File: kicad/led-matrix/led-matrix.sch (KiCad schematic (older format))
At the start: 4 parts

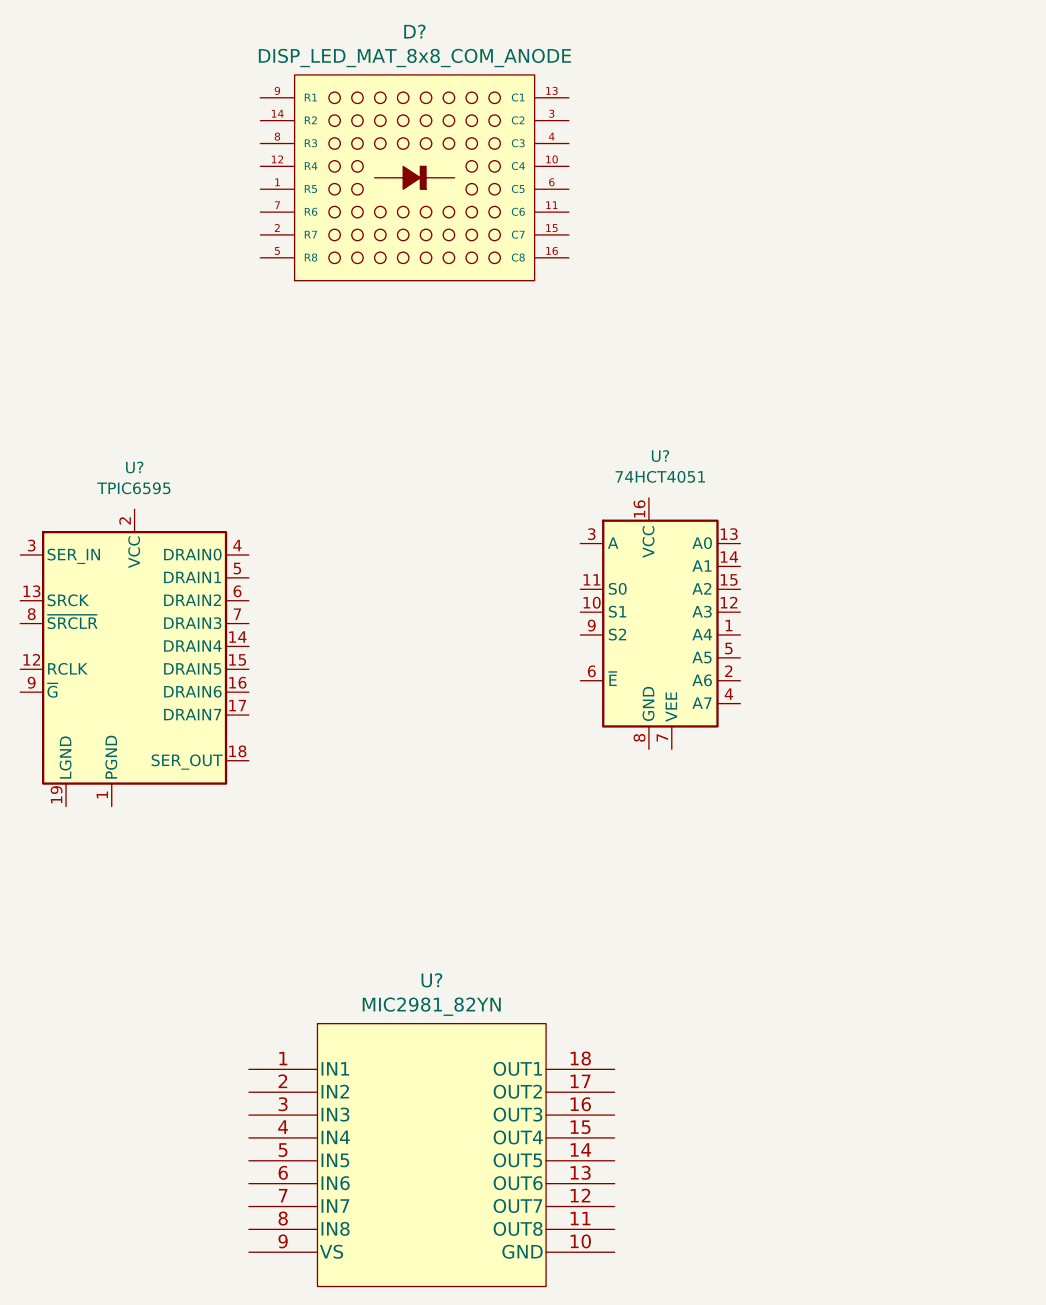
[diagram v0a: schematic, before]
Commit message: Update schematix
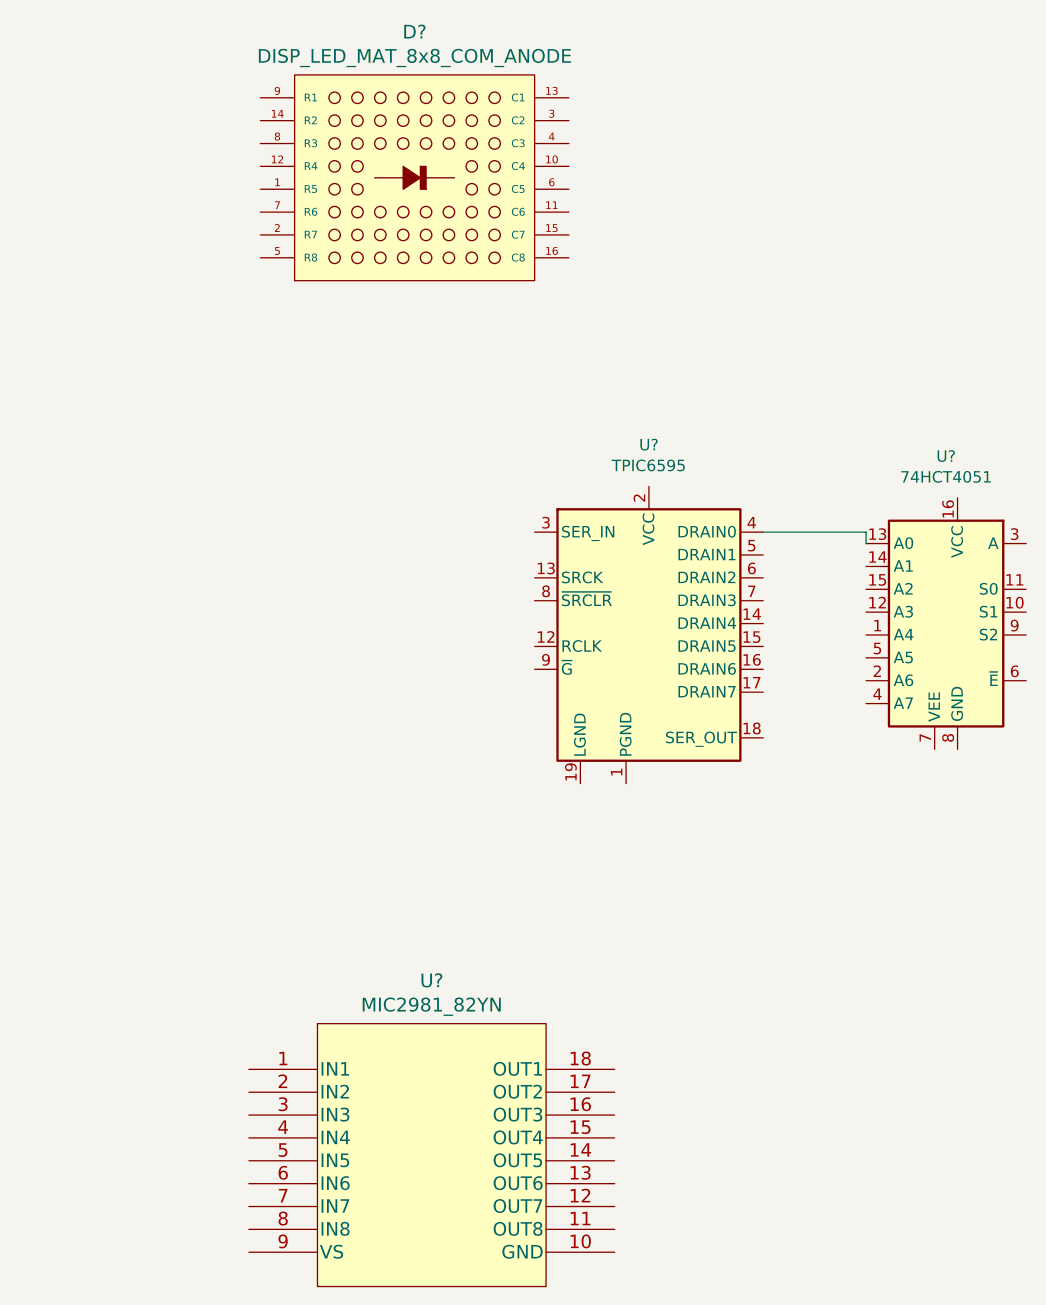
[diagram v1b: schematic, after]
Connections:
- net at U?.4 (DRAIN0): now also U?.13 (A0)
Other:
- moved on the sheet: U?
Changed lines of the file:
@@
 $EndDescr
-$Comp
-L Interface_Expansion:TPIC6595 U?
-U 1 1 5FD7CD50
-P 5150 3100
-F 0 "U?" H 5150 3881 50  0000 C CNN
-F 1 "TPIC6595" H 5150 3790 50  0000 C CNN
-F 2 "" H 5800 2450 50  0001 C CNN
-F 3 "http://www.ti.com/lit/ds/symlink/tpic6595.pdf" H 5150 3050 50  0001 C CNN
-	1    5150 3100
-	1    0    0    -1
-$EndComp
-$Comp
-L 74xx:74HCT4051 U?
-U 1 1 5FD7E6DB
-P 7400 2950
-F 0 "U?" H 7450 3631 50  0000 C CNN
-F 1 "74HCT4051" H 7450 3540 50  0000 C CNN
-F 2 "" H 7400 2550 50  0001 C CNN
-F 3 "http://www.ti.com/lit/ds/symlink/cd74hct4051.pdf" H 7400 2550 50  0001 C CNN
-	1    7400 2950
-	1    0    0    -1
-$EndComp
 $Comp
 L MIC2981:MIC2981_82YN U?
@@
 	1    0    0    -1
 $EndComp
+Wire Wire Line
+	7900 2600 8350 2600
+Wire Wire Line
+	8350 2600 8350 2650
+$Comp
+L 74xx:74HCT4051 U?
+U 1 1 5FD7E6DB
+P 8750 2950
+F 0 "U?" H 8800 3631 50  0000 C CNN
+F 1 "74HCT4051" H 8800 3540 50  0000 C CNN
+F 2 "" H 8750 2550 50  0001 C CNN
+F 3 "http://www.ti.com/lit/ds/symlink/cd74hct4051.pdf" H 8750 2550 50  0001 C CNN
+	1    8750 2950
+	-1   0    0    -1
+$EndComp
+$Comp
+L Interface_Expansion:TPIC6595 U?
+U 1 1 5FD7CD50
+P 7400 3000
+F 0 "U?" H 7400 3781 50  0000 C CNN
+F 1 "TPIC6595" H 7400 3690 50  0000 C CNN
+F 2 "" H 8050 2350 50  0001 C CNN
+F 3 "http://www.ti.com/lit/ds/symlink/tpic6595.pdf" H 7400 2950 50  0001 C CNN
+	1    7400 3000
+	1    0    0    -1
+$EndComp
